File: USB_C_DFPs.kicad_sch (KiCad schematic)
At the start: 34 parts, among them J5 USB_C_Receptacle, J6 USB_C_Receptacle, Q5 IRF7807, U6 LM3478MM_NOPB, U7 SY6280, U8 SY6280

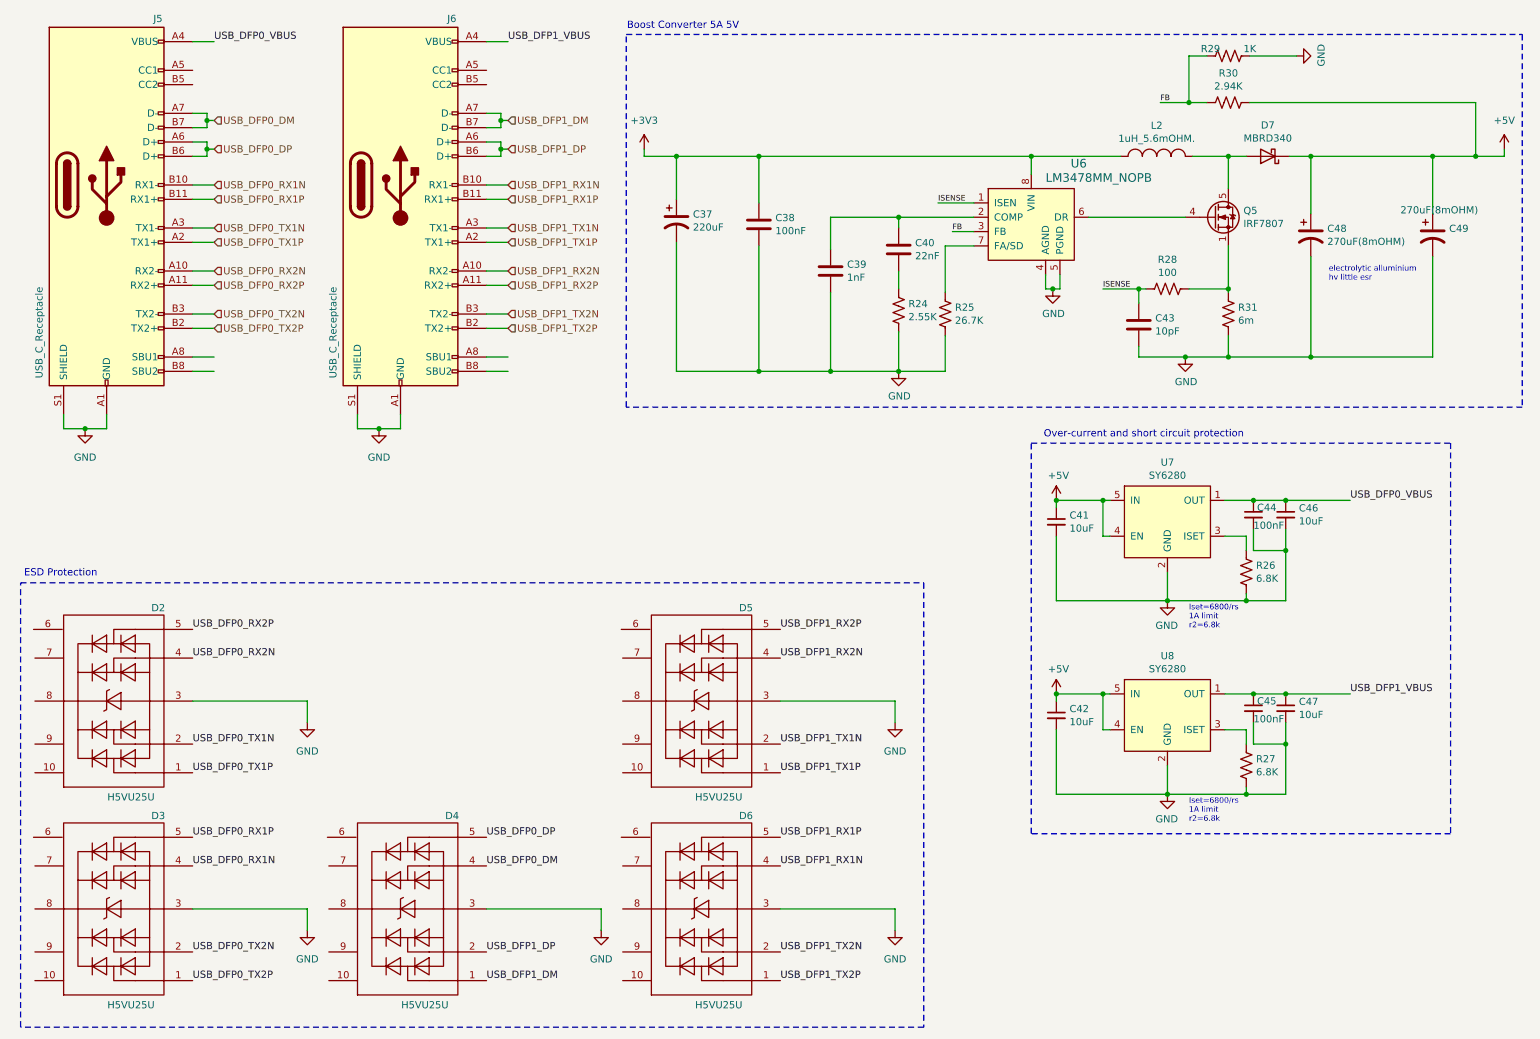
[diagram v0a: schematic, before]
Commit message: Updated schematics
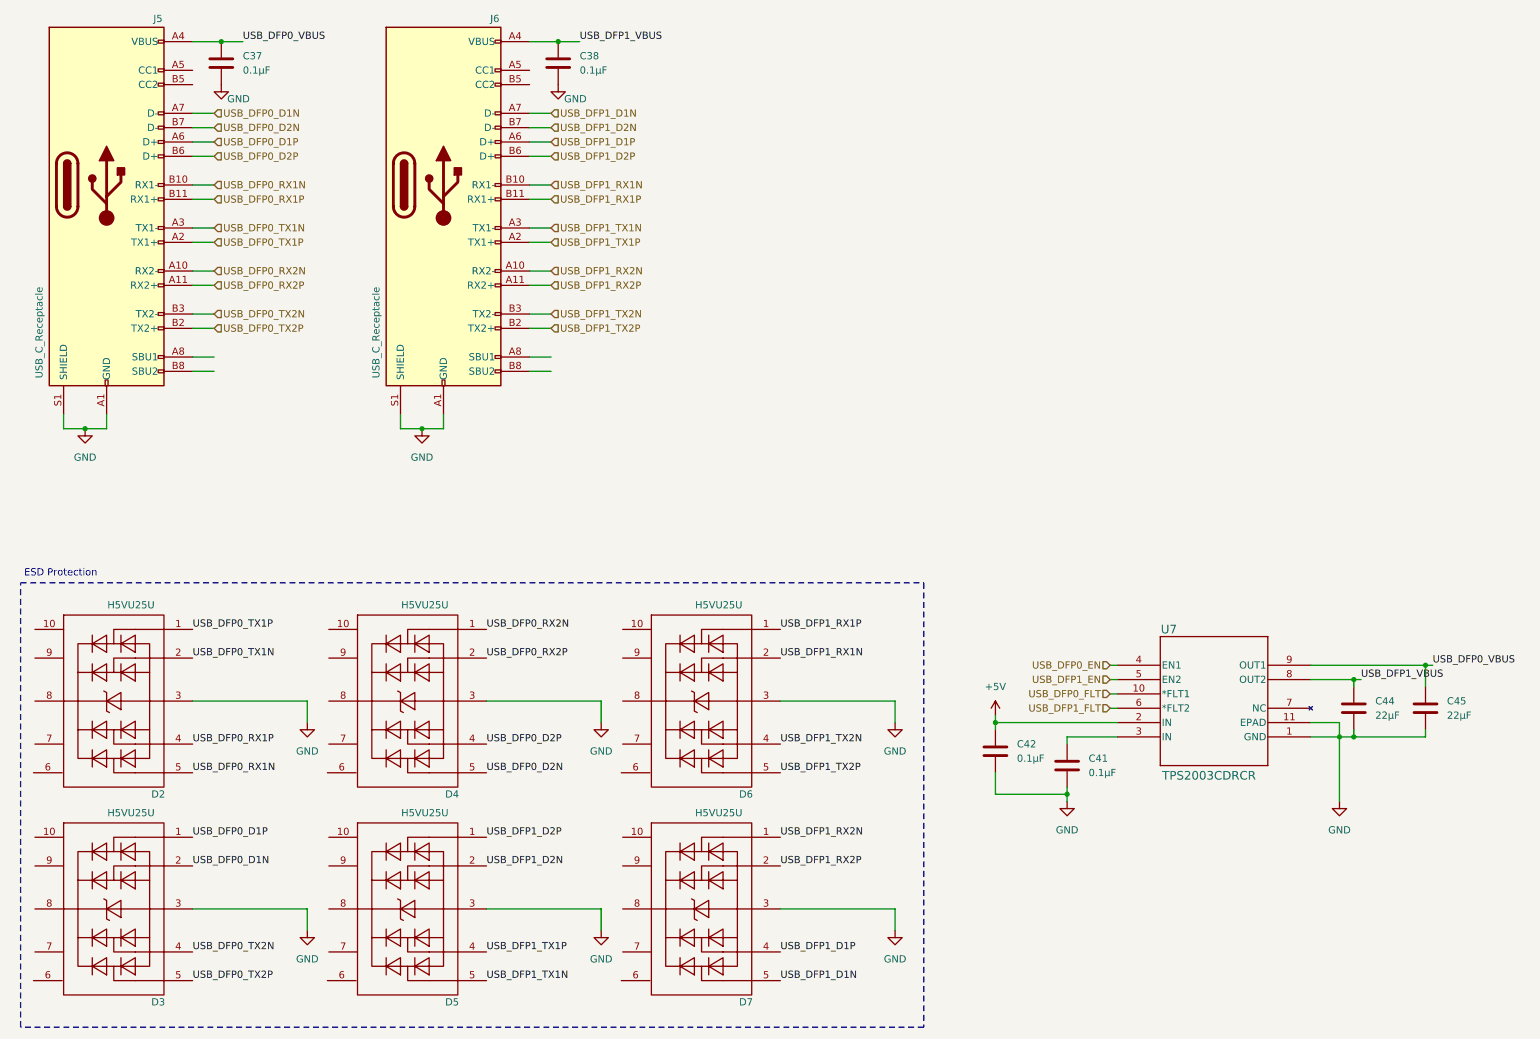
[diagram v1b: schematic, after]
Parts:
- removed C37: 220uF, Capacitor_SMD:CP_Elec_10x10, symbol USB_C_HUB-rescue:CP1-Device
- removed C39: 1nF, Capacitor_SMD:C_0402_1005Metric, symbol Device:C
- removed C40: 22nF, Capacitor_SMD:C_0402_1005Metric, symbol Device:C
- removed C41, C42, C46, C47: 10uF, Capacitor_SMD:C_0603_1608Metric, symbol Device:C_Small
- removed C43: 10pF, Capacitor_SMD:C_0402_1005Metric, symbol Device:C
- removed C44, C45: 100nF, Capacitor_SMD:C_0402_1005Metric, symbol Device:C_Small
- removed C48, C49: 270uF(8mOHM), Capacitor_THT:CP_Radial_D8.0mm_P3.50mm, symbol USB_C_HUB-rescue:CP1-Device
- removed D7: MBRD340, SamacSys_Parts_2:STPS30L30DJFTR, symbol Device:D_Schottky
- removed L2: 1uH_5.6mOHM., Inductor_SMD:L_Sunlord_MWSA1004S, symbol USB_C_HUB-rescue:INDUCTOR_SMALL-OLIMEX_RCL
- removed Q5: IRF7807, symbol Transistor_FET:CSD17579Q5A
- removed R24: 2.55K, Resistor_SMD:R_0603_1608Metric, symbol Device:R_US
- removed R25: 26.7K, Resistor_SMD:R_0603_1608Metric, symbol Device:R_US
- removed R26, R27: 6.8K, Resistor_SMD:R_0603_1608Metric, symbol Device:R_US
- removed R28: 100, Resistor_SMD:R_0603_1608Metric, symbol Device:R_US
- removed R29: 1K, Resistor_SMD:R_0603_1608Metric, symbol Device:R_US
- removed R30: 2.94K, Resistor_SMD:R_0603_1608Metric, symbol Device:R_US
- removed R31: 6m, Resistor_SMD:R_0805_2012Metric, symbol Device:R_US
- removed U6: LM3478MM_NOPB, digikey-footprints:TSSOP-8_W3mm, symbol USB_C_HUB-rescue:LM3478MM_NOPB-dk_PMIC-Voltage-Regulators-DC-DC-Switching-Contr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
- removed U7, U8: SY6280, Package_TO_SOT_SMD:SOT-23-5, symbol USB_C_HUB-rescue:SY6280-usb_hub
- added C37, C41, C42: 0.1μF, Capacitor_SMD:C_0402_1005Metric, symbol Device:C
- added C44, C45: 22μF, Capacitor_SMD:C_0603_1608Metric, symbol Device:C
- added D4: H5VU25U, AZ1045-04F:AZ1045-04F, symbol AZ1045-04F:AZ1045-04F
- added U7: TPS2003CDRCR, DRC10_1P65X2P40_TEX, symbol TPS2003CDRCR:TPS2003CDRCR
- C38: value 100nF -> 0.1μF; LCSC C60474 -> C1525; Part_Number CC0402KRX7R7BB104 -> CL05B104KO5NNNC
- D2, D3: footprint kicad_lceda:DFN2510-10_L2.5-W1.0-P0.50-BL -> AZ1045-04F:AZ1045-04F
- D5: renamed from D4; footprint kicad_lceda:DFN2510-10_L2.5-W1.0-P0.50-BL -> AZ1045-04F:AZ1045-04F
- D6: renamed from D5; footprint kicad_lceda:DFN2510-10_L2.5-W1.0-P0.50-BL -> AZ1045-04F:AZ1045-04F
- D7: renamed from D6; footprint kicad_lceda:DFN2510-10_L2.5-W1.0-P0.50-BL -> AZ1045-04F:AZ1045-04F
- J5, J6: footprint (none) -> USB-C-SMD_TYPE-C-24P-QT:USB-C-SMD_TYPE-C-24P-QT; LCSC (none) -> C2681555; Part_Number (none) -> TYPE-C 24P QT
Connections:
- net +3V3 is gone; now on net USB_DFP1_VBUS: C38.1
- net +5V: now also C42.1, U7.2 (IN)
- net GND: now also C37.2, C41.2, C42.2, C44.2, C45.2, D4.3 (GND), U7.1 (GND), U7.11 (EPAD)
- net USB_DFP0_RX1N: now also D2.5 (I/O_4); no longer D3.4 (I/O_3)
- net USB_DFP0_RX1P: now also D2.4 (I/O_3); no longer D3.5 (I/O_4)
- net USB_DFP0_RX2N: now also D4.1 (I/O_1); no longer D2.4 (I/O_3)
- net USB_DFP0_RX2P: now also D4.2 (I/O_2); no longer D2.5 (I/O_4)
- net USB_DFP0_TX2N: now also D3.4 (I/O_3); no longer D3.2 (I/O_2)
- net USB_DFP0_TX2P: now also D3.5 (I/O_4); no longer D3.1 (I/O_1)
- net USB_DFP0_VBUS: now also C37.1, C45.1, U7.9 (OUT1)
- net USB_DFP1_RX1N: now also D6.2 (I/O_2); no longer D7.4 (I/O_3)
- net USB_DFP1_RX1P: now also D6.1 (I/O_1); no longer D7.5 (I/O_4)
- net USB_DFP1_RX2N: now also D7.1 (I/O_1); no longer D6.4 (I/O_3)
- net USB_DFP1_RX2P: now also D7.2 (I/O_2); no longer D6.5 (I/O_4)
- net USB_DFP1_TX1N: now also D5.5 (I/O_4); no longer D6.2 (I/O_2)
- net USB_DFP1_TX1P: now also D5.4 (I/O_3); no longer D6.1 (I/O_1)
- net USB_DFP1_TX2N: now also D6.4 (I/O_3); no longer D7.2 (I/O_2)
- net USB_DFP1_TX2P: now also D6.5 (I/O_4); no longer D7.1 (I/O_1)
- net USB_DFP1_VBUS: now also C44.1, U7.8 (OUT2)
- removed net USB_DFP0_DM: D5.4 (I/O_3), J5.A7 (D-), J5.B7 (D-)
- removed net USB_DFP0_DP: D5.5 (I/O_4), J5.A6 (D+), J5.B6 (D+)
- removed net USB_DFP1_DM: D5.1 (I/O_1), J6.A7 (D-), J6.B7 (D-)
- removed net USB_DFP1_DP: D5.2 (I/O_2), J6.A6 (D+), J6.B6 (D+)
- new net: C41.1, U7.3 (IN)
- new net USB_DFP0_D1N: D3.2 (I/O_2), J5.A7 (D-)
- new net USB_DFP0_D1P: D3.1 (I/O_1), J5.A6 (D+)
- new net USB_DFP0_D2N: D4.5 (I/O_4), J5.B7 (D-)
- new net USB_DFP0_D2P: D4.4 (I/O_3), J5.B6 (D+)
- new net USB_DFP0_EN: U7.4 (EN1)
- new net USB_DFP0_FLT: U7.10 (*FLT1)
- new net USB_DFP1_D1N: D7.5 (I/O_4), J6.A7 (D-)
- new net USB_DFP1_D1P: D7.4 (I/O_3), J6.A6 (D+)
- new net USB_DFP1_D2N: D5.2 (I/O_2), J6.B7 (D-)
- new net USB_DFP1_D2P: D5.1 (I/O_1), J6.B6 (D+)
- new net USB_DFP1_EN: U7.5 (EN2)
- new net USB_DFP1_FLT: U7.6 (*FLT2)
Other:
- note removed: "Boost Converter 5A 5V"
- note removed: "Iset=6800/rs 1A limit r2=6.8k"
- note removed: "Over-current and short circuit protection"
- note removed: "electrolytic alluminium hv little esr"
- moved on the sheet: J6

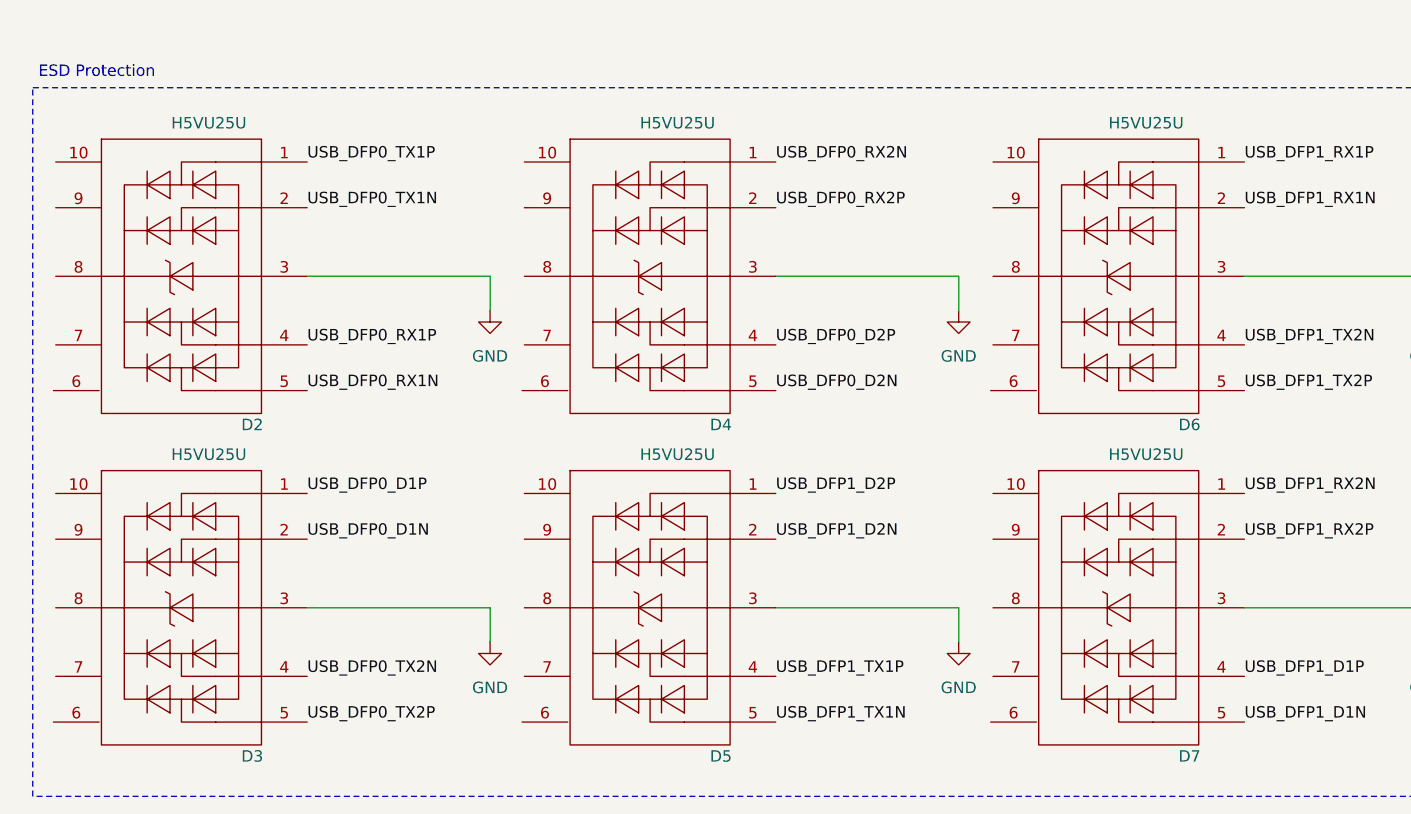
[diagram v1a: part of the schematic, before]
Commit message: Continue working on board layout
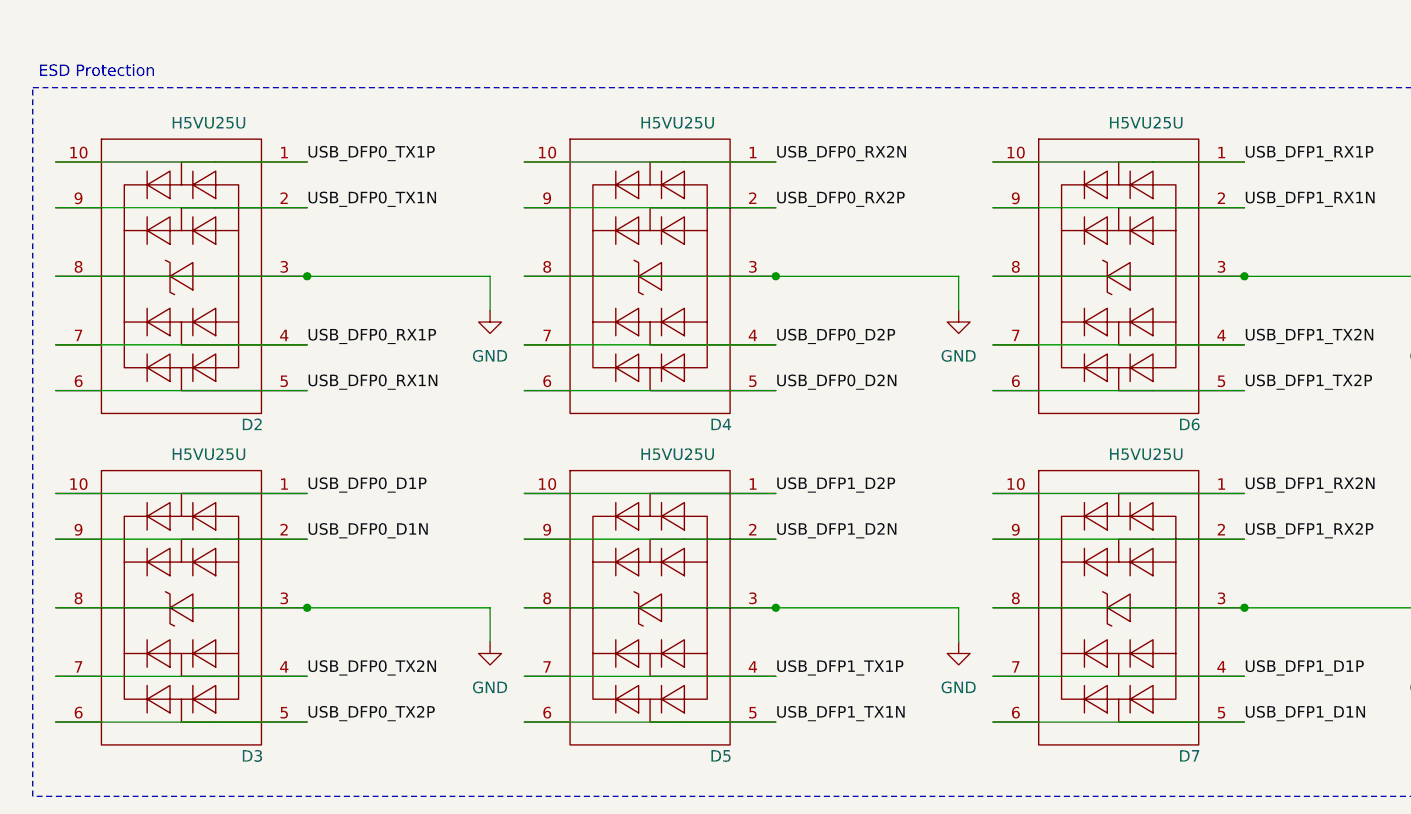
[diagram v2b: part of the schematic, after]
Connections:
- net GND: now also D2.8 (GND), D3.8 (GND), D4.8 (GND), D5.8 (GND), D6.8 (GND), D7.8 (GND)
- net USB_DFP0_D1N: now also D3.9 (NC)
- net USB_DFP0_D1P: now also D3.10 (NC)
- net USB_DFP0_D2N: now also D4.6 (NC)
- net USB_DFP0_D2P: now also D4.7 (NC)
- net USB_DFP0_RX1N: now also D2.6 (NC)
- net USB_DFP0_RX1P: now also D2.7 (NC)
- net USB_DFP0_RX2N: now also D4.10 (NC)
- net USB_DFP0_RX2P: now also D4.9 (NC)
- net USB_DFP0_TX1N: now also D2.9 (NC)
- net USB_DFP0_TX1P: now also D2.10 (NC)
- net USB_DFP0_TX2N: now also D3.7 (NC)
- net USB_DFP0_TX2P: now also D3.6 (NC)
- net USB_DFP1_D1N: now also D7.6 (NC)
- net USB_DFP1_D1P: now also D7.7 (NC)
- net USB_DFP1_D2N: now also D5.9 (NC)
- net USB_DFP1_D2P: now also D5.10 (NC)
- net USB_DFP1_RX1N: now also D6.9 (NC)
- net USB_DFP1_RX1P: now also D6.10 (NC)
- net USB_DFP1_RX2N: now also D7.10 (NC)
- net USB_DFP1_RX2P: now also D7.9 (NC)
- net USB_DFP1_TX1N: now also D5.6 (NC)
- net USB_DFP1_TX1P: now also D5.7 (NC)
- net USB_DFP1_TX2N: now also D6.7 (NC)
- net USB_DFP1_TX2P: now also D6.6 (NC)
